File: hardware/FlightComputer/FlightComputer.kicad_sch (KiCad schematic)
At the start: 79 parts, among them IC1 TPS54295PWPR, IC2 LM75AD,118, IC3 LM75AD,118, IC4 LM75AD,118, J1 Screw_Terminal_01x02, J10 Conn_01x20_Male, J2 SWD, J3 USB_B_Micro, J4 IMU, J5 L77TSAH15SOL2RM8, J6 Mag, J7 Camera, J8 Conn_01x20_Male, U1 SN74LVC2G04DCKR, U2 STM32F103VCT6, U3 USBLC6-2SC6, Y1 ABM3B-8.000MHZ-10-1-U-T

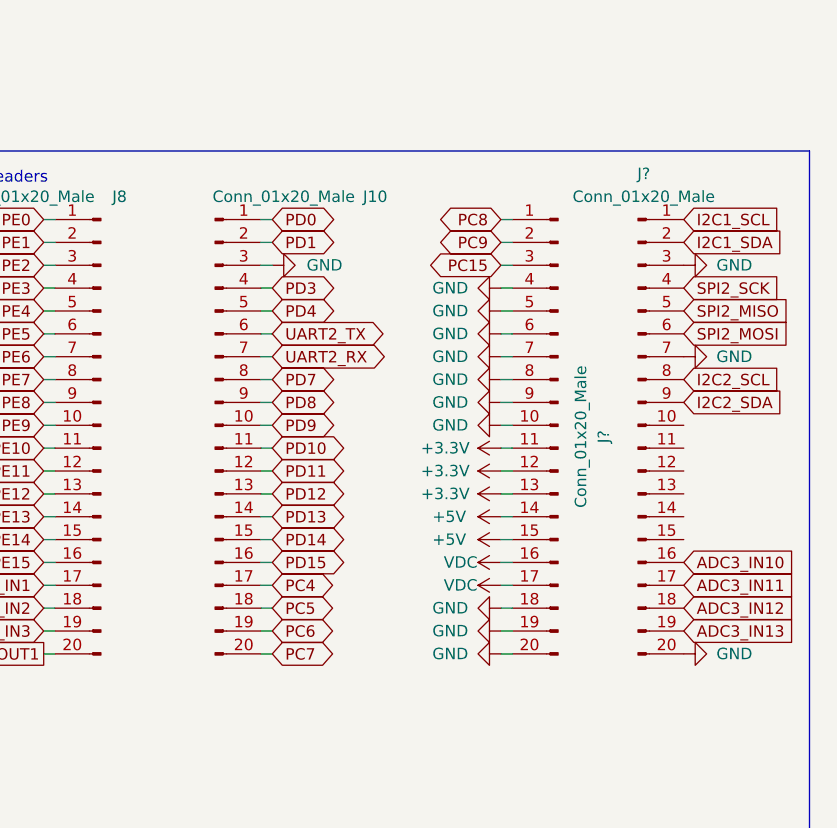
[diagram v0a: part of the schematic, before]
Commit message: Update FlightComputer.kicad_sch
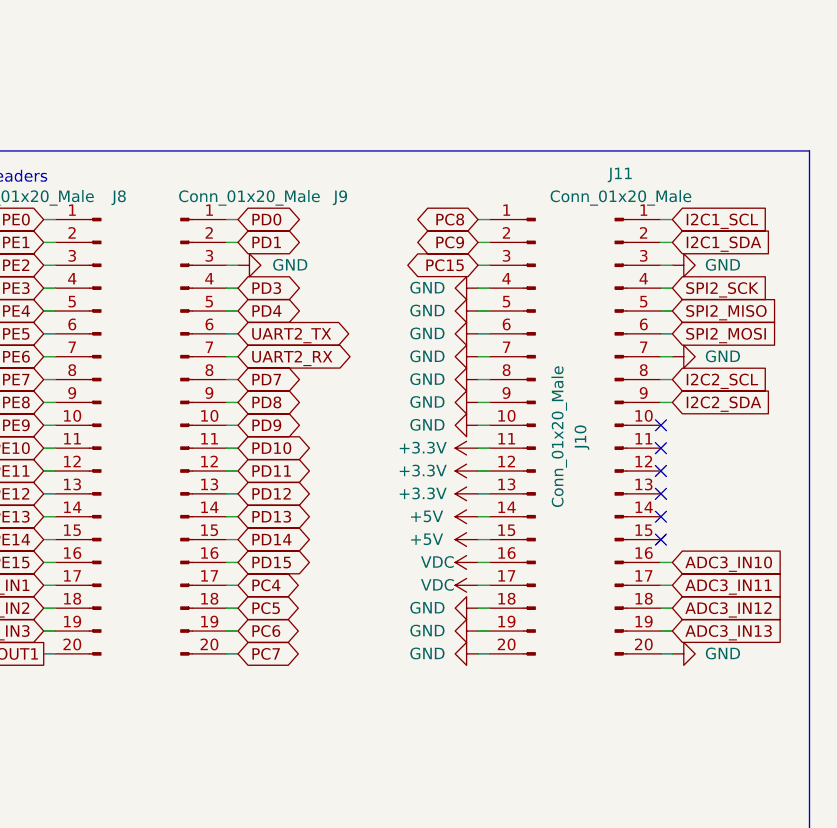
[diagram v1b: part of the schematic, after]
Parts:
- gave numbers to parts that had none: 2
- renumbered J10 to J9
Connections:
- no-connect marks 11 -> 17
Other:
- moved on the sheet: J10, J11, J9
